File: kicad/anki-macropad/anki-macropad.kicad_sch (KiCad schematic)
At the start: 46 parts, among them J1 USB_C_Receptacle_USB2.0_14P, SW1 PTS810 SJK 250 SMTR LFS, U1 NCP1117-3.3_SOT223, U2 W25Q128JVS, U3 RP2040, U4 USBLC6-2SC6, X1 ABM8-272-T3

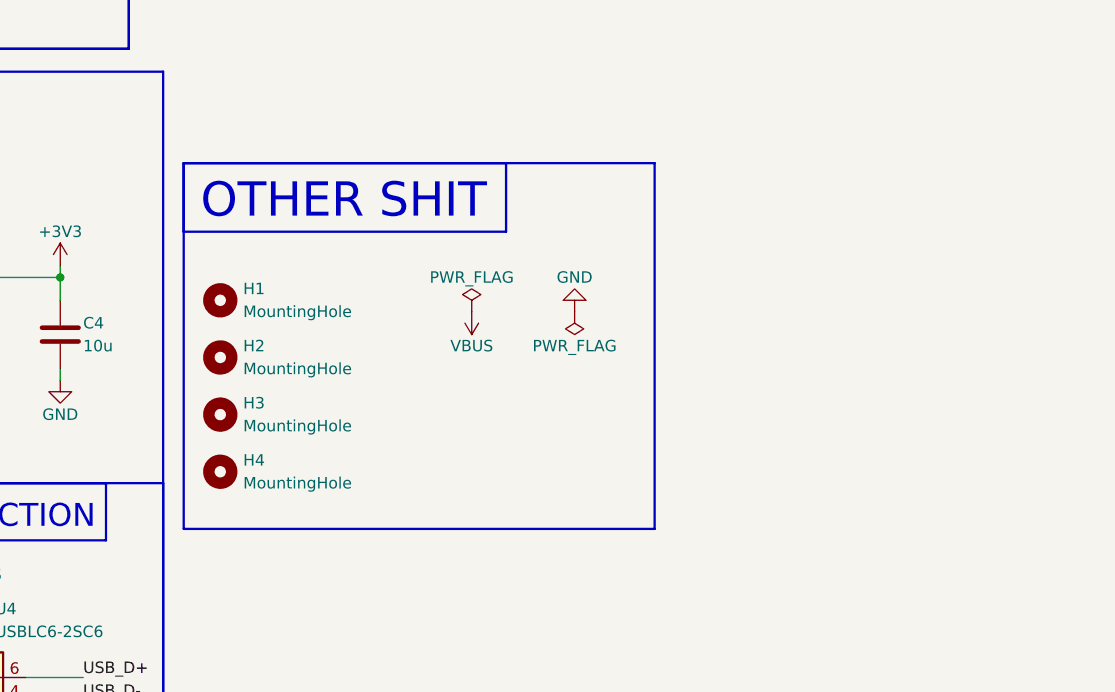
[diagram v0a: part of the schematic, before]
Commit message: Pretty much finished the PCB. Just need to go through DRC.
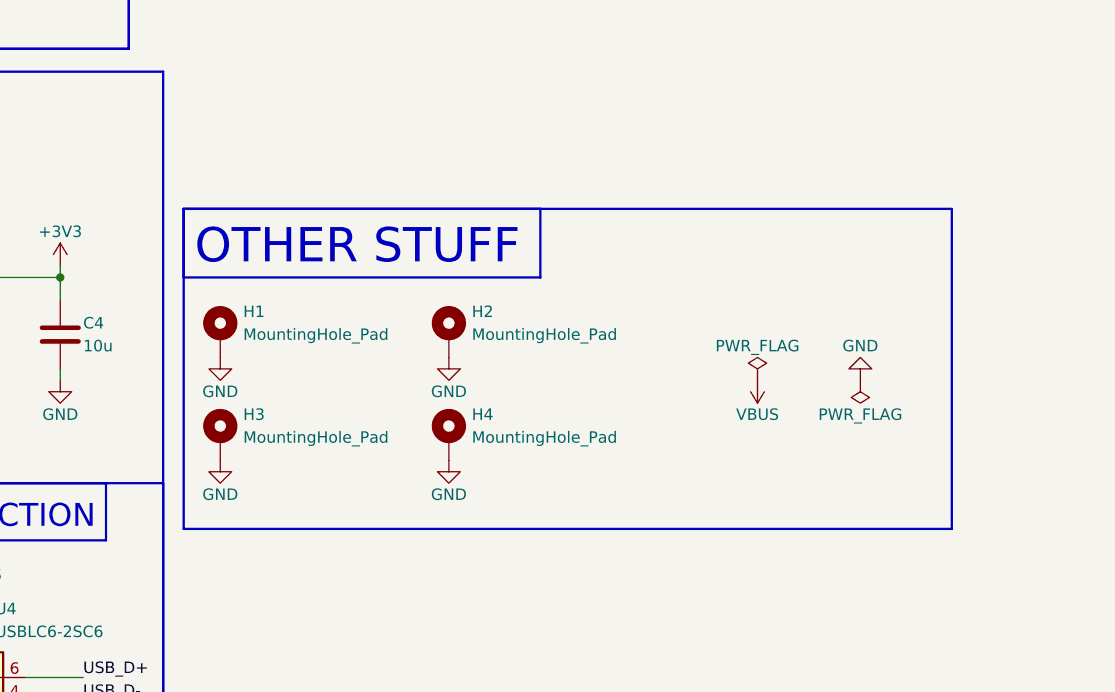
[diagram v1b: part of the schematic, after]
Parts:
- removed H1, H2, H3, H4: MountingHole, MountingHole:MountingHole_2.7mm_M2.5, symbol Mechanical:MountingHole
- added H1, H2, H3, H4: MountingHole_Pad, MountingHole:MountingHole_2.7mm_M2.5_Pad, symbol Mechanical:MountingHole_Pad
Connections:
- net GND: now also H1.1, H2.1, H3.1, H4.1
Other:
- note added: "OTHER STUFF"
- note removed: "OTHER SHIT"
